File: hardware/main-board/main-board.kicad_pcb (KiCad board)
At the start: 2 copper layers, 48 x 48 mm, 44 parts, among them J1 USB-C Receptacle, J2 JST JWPF, J3 LCD_FFC_SOLDER, Q1 SS8050-G, Q2 SS8050-G, Q3 SS8050-G, SW1 FRONT_BUTTON, U1 SN65HVD230, U2 CPC1017N, U3 AP1509-33SG-13, U4 CP2102N-A01-GQFN28, U5 ESP32-WROOM-32

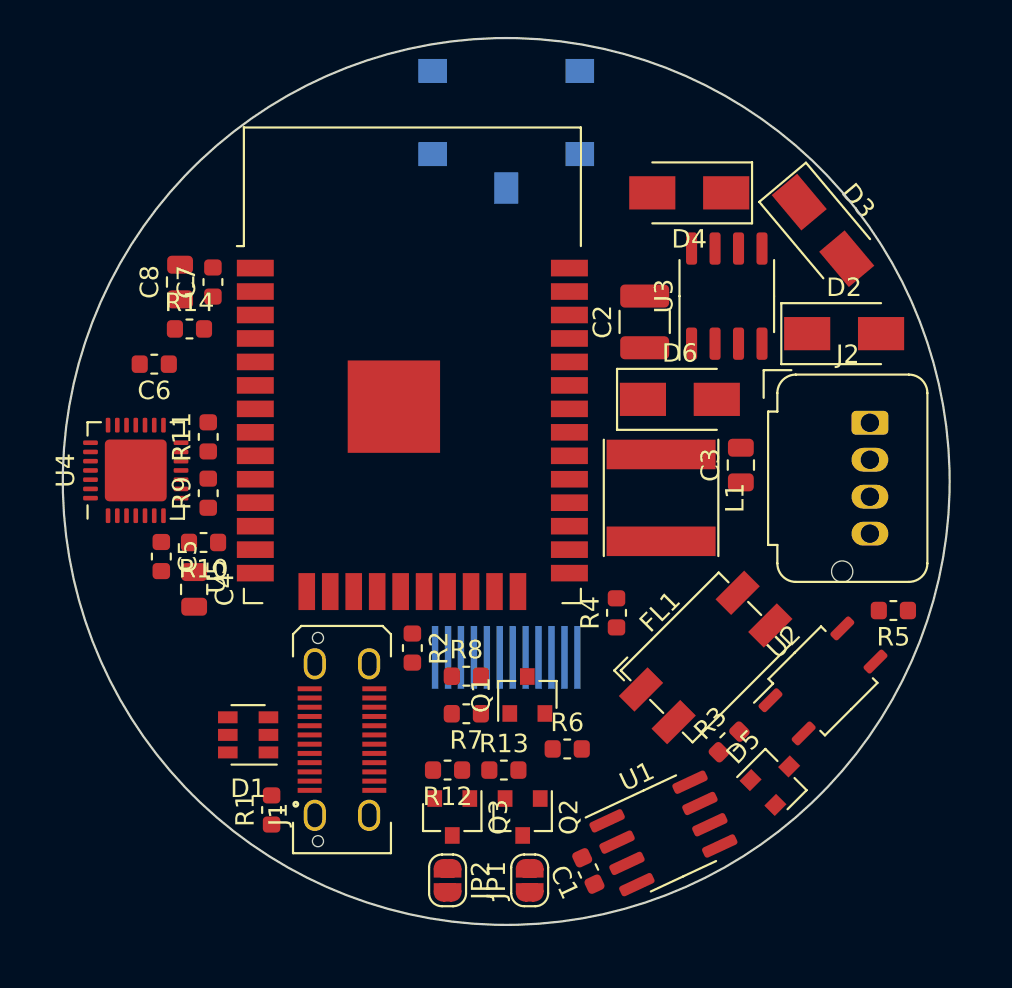
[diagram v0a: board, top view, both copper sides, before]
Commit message: layout almost done
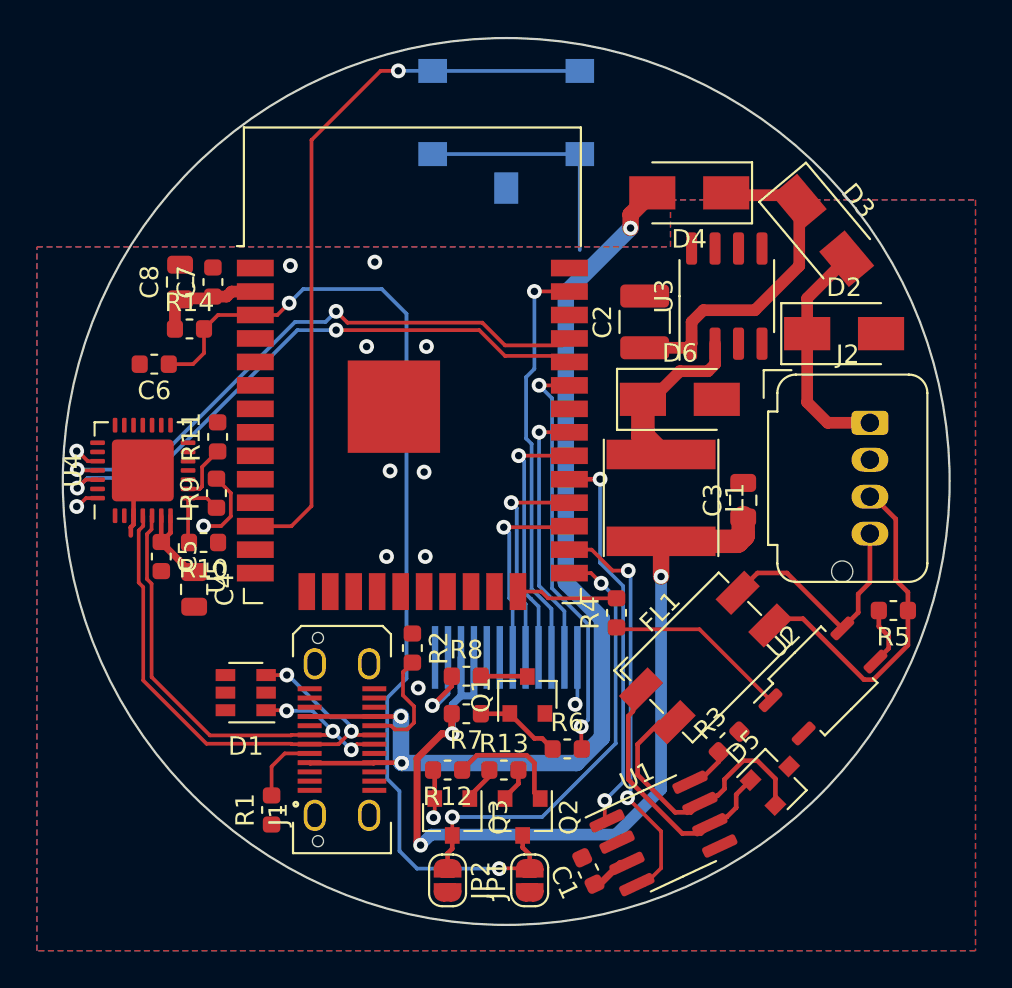
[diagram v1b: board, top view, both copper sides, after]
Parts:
- moved D1 2.29 mm to (-14.1, 11.4)
- moved C3 1.91 mm to (12.8, 1.02)
- moved R11 0.51 mm to (-15.6, -2.41)
- moved R9 0.44 mm to (-15.7, 0.64)
- moved U4 0.38 mm to (-19.7, -0.60)
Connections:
- D1 pad 1: /USB_D+ -> /USB_D-
- D1 pad 3: /USB_D- -> /USB_D+
- R4 pad 2: (no net) -> /ESP32/CANBUS_TERM_EN
- U5 pad 24: (no net) -> /ESP32/CANBUS_TERM_EN
- U5 pad 39: (no net) -> GND
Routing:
- net +3V3: track 0.00 -> 62.4 mm, vias 0 -> 3
- net /USB_VBUS: track 0.00 -> 60.2 mm, vias 0 -> 4
- net /ESP32/EN: track 0.00 -> 55.0 mm, vias 0 -> 2
- net /ESP32/FRONT_BUTTON: track 0.00 -> 39.4 mm, vias 0 -> 1
- net /ESP32/PROG_TXD: track 0.00 -> 32.2 mm, vias 0 -> 2
- net /ESP32/PROG_RX: track 0.00 -> 32.2 mm, vias 0 -> 2
- net /USB_D+: track 0.00 -> 29.5 mm, vias 0 -> 2
- net /USB_D-: track 0.00 -> 27.0 mm, vias 0 -> 3
- net /ESP32/IO0: track 0.00 -> 24.3 mm, vias 0 -> 2
- net /LCD/BACKLIGHT: track 0.00 -> 22.6 mm, vias 0 -> 2
- net /ESP32/LCD_SDO: track 0.00 -> 22.5 mm, vias 0 -> 1
- net /ESP32/CANBUS_TX: track 0.00 -> 22.3 mm, vias 0 -> 2
- net /ESP32/CANBUS_RX: track 0.00 -> 21.1 mm, vias 0 -> 2
- net GND: track 0.00 -> 19.5 mm, vias 0 -> 10
- net /CANH: track 0.00 -> 18.7 mm
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- added copper zone on B.Cu, net GND
- added copper zone on F.Cu, net GND
